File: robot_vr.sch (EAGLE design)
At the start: 34 parts, among them CN10 SSM-119-L-DV, CN7 SSM-119-L-DV

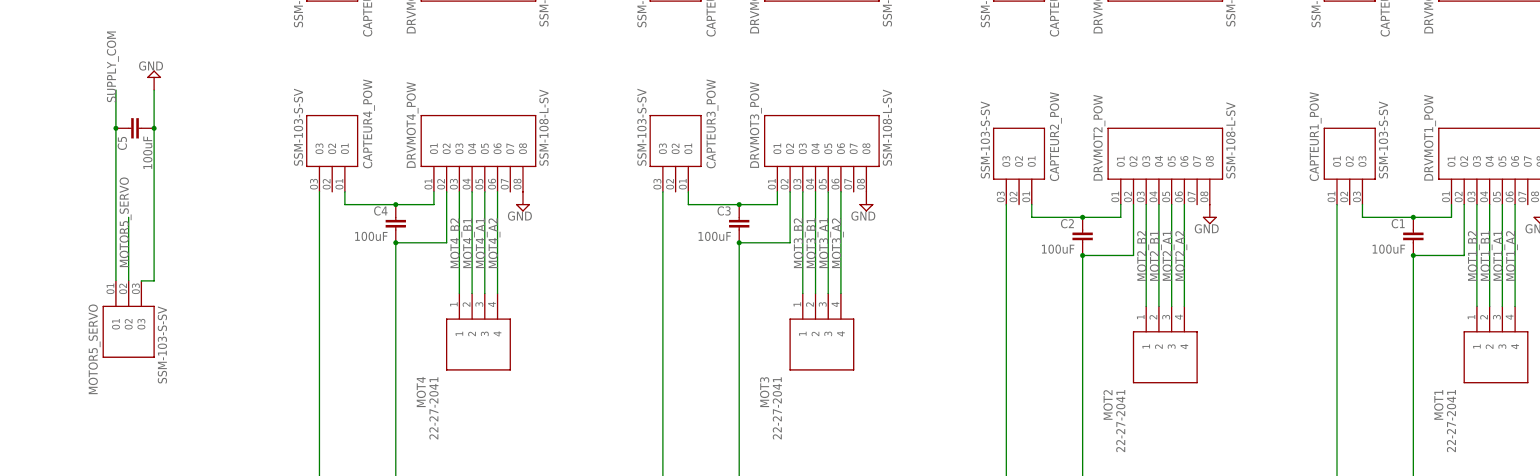
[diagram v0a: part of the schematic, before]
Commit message: Add files via upload
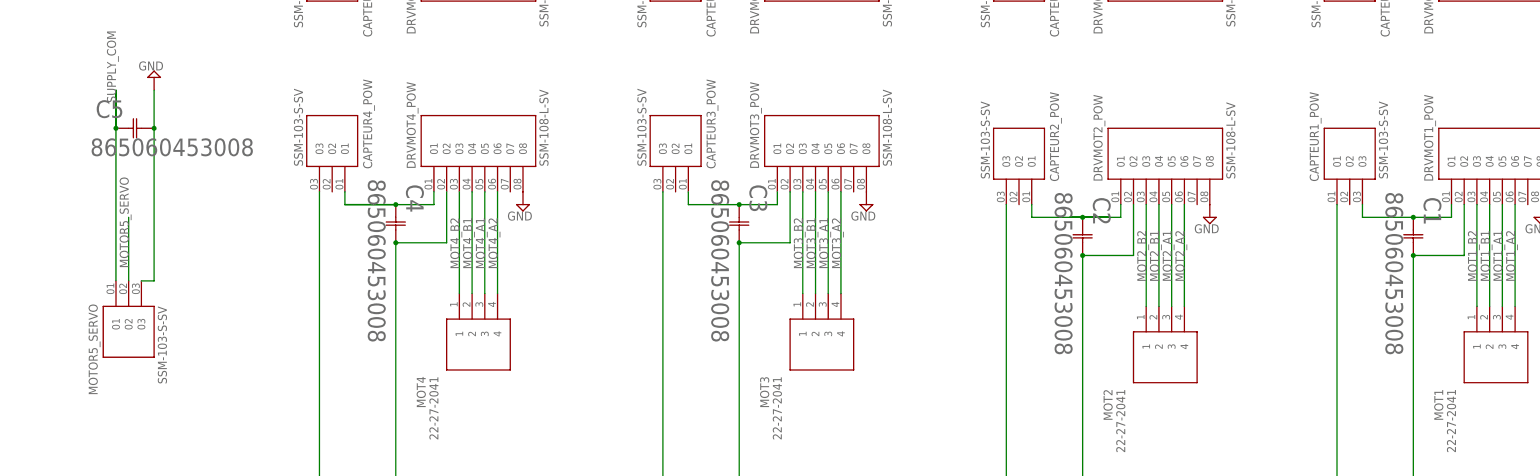
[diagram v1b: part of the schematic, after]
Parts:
- C1, C2, C3, C4, C5: value 100uF -> 865060453008; device rcl:C-EUC1206K -> Condo-Wurth:865060453008
